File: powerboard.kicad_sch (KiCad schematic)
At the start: 27 parts, among them J1 B03B, J2 EMER_SW, J3 EMER_SW, Q1 TJ60S04M3L, U1 PQQ10W-Q24-S5-S, U2 TLP222A

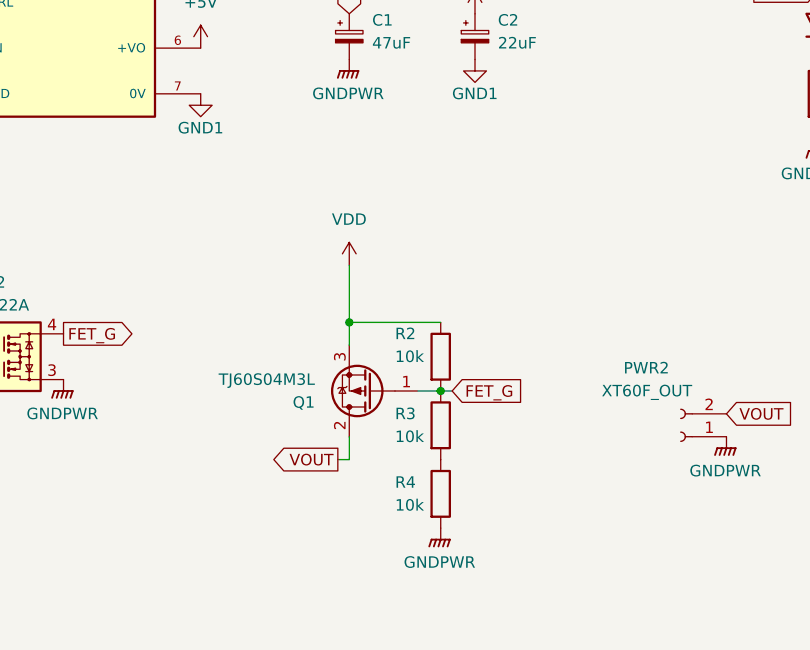
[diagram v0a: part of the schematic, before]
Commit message: ツェナーで定電圧チャレンジ
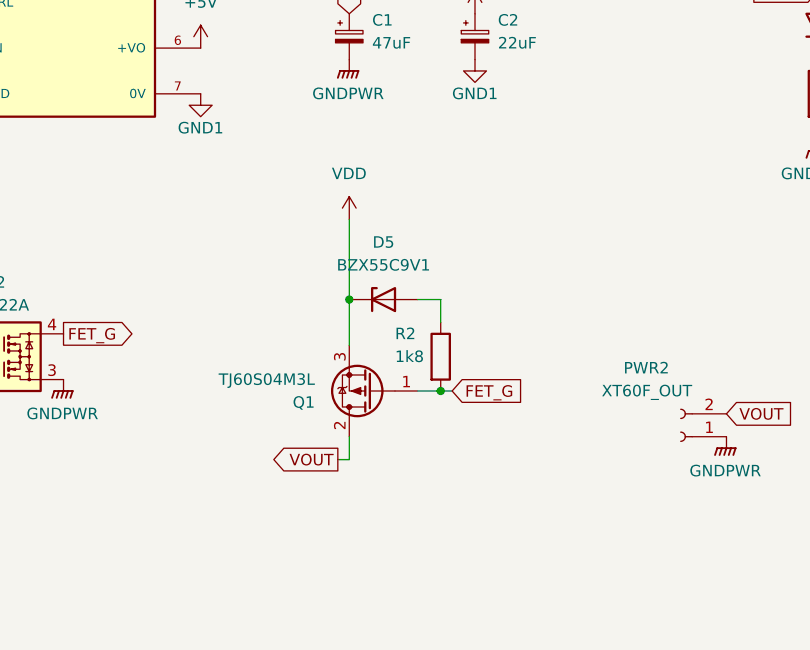
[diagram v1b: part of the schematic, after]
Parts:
- removed R3, R4: 10k, Resistor_THT:R_Axial_DIN0207_L6.3mm_D2.5mm_P7.62mm_Horizontal, symbol Device:R
- added D5: BZX55C9V1, Diode_THT:D_DO-35_SOD27_P10.16mm_Horizontal, symbol Diode:ZPDxx
- R2: value 10k -> 1k8
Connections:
- net VDD: now also D5.1 (K); no longer R2.1
- new net: D5.2 (A), R2.1
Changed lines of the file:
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@@
 	(paper "A4")
+	(junction
+		(at 144.78 66.04)
+		(diameter 0)
+		(color 0 0 0 0)
+	)
 	(junction
 		(at 154.94 76.2)
@@
 		(color 0 0 0 0)
 	)
-	(junction
-		(at 144.78 68.58)
-		(diameter 0)
-		(color 0 0 0 0)
-	)
 	(no_connect
 		(at 97.79 33.02)
@@
 	(wire
 		(pts
-			(xy 144.78 62.23) (xy 144.78 68.58)
+			(xy 144.78 57.15) (xy 144.78 66.04)
 		)
 		(stroke
@@
 	(wire
 		(pts
-			(xy 144.78 68.58) (xy 144.78 71.12)
+			(xy 55.88 41.91) (xy 39.37 41.91)
 		)
 		(stroke
@@
 	(wire
 		(pts
-			(xy 55.88 41.91) (xy 39.37 41.91)
+			(xy 67.31 69.85) (xy 80.01 69.85)
 		)
 		(stroke
@@
 	(wire
 		(pts
-			(xy 67.31 69.85) (xy 80.01 69.85)
+			(xy 82.55 69.85) (xy 86.36 69.85)
 		)
 		(stroke
@@
 	(wire
 		(pts
-			(xy 82.55 69.85) (xy 86.36 69.85)
+			(xy 96.52 38.1) (xy 97.79 38.1)
 		)
 		(stroke
@@
 	(wire
 		(pts
-			(xy 96.52 38.1) (xy 97.79 38.1)
+			(xy 97.79 74.93) (xy 97.79 77.47)
 		)
 		(stroke
@@
 	(wire
 		(pts
-			(xy 97.79 74.93) (xy 97.79 77.47)
+			(xy 60.96 39.37) (xy 59.69 39.37)
 		)
 		(stroke
@@
 	(wire
 		(pts
-			(xy 60.96 39.37) (xy 59.69 39.37)
+			(xy 25.4 71.12) (xy 33.02 71.12)
 		)
 		(stroke
@@
 	(wire
 		(pts
-			(xy 25.4 71.12) (xy 33.02 71.12)
+			(xy 55.88 41.91) (xy 55.88 43.18)
 		)
 		(stroke
@@
 	(wire
 		(pts
-			(xy 55.88 41.91) (xy 55.88 43.18)
+			(xy 144.78 83.82) (xy 144.78 81.28)
 		)
 		(stroke
@@
 	(wire
 		(pts
-			(xy 144.78 83.82) (xy 144.78 81.28)
+			(xy 156.21 76.2) (xy 154.94 76.2)
 		)
 		(stroke
@@
 	(wire
 		(pts
-			(xy 156.21 76.2) (xy 154.94 76.2)
+			(xy 96.52 44.45) (xy 96.52 43.18)
 		)
 		(stroke
@@
 	(wire
 		(pts
-			(xy 96.52 44.45) (xy 96.52 43.18)
+			(xy 152.4 66.04) (xy 154.94 66.04)
 		)
 		(stroke
@@
 	(wire
 		(pts
-			(xy 144.78 68.58) (xy 154.94 68.58)
+			(xy 144.78 66.04) (xy 144.78 71.12)
 		)
 		(stroke
@@
 		)
 	)
+	(wire
+		(pts
+			(xy 154.94 66.04) (xy 154.94 68.58)
+		)
+		(stroke
+			(width 0)
+			(type default)
+		)
+	)
 	(global_label "sig"
 		(shape input)
@@
 	)
 	(symbol
-		(lib_id "power:GNDPWR")
-		(at 154.94 91.44 0)
-		(unit 1)
-		(exclude_from_sim no)
-		(in_bom yes)
-		(on_board yes)
-		(dnp no)
-		(fields_autoplaced yes)
-		(property "Reference" "#PWR012"
-			(at 154.94 96.52 0)
-			(effects
-				(font
-					(size 1.27 1.27)
-				)
-				(hide yes)
-			)
-		)
-		(property "Value" "GNDPWR"
-			(at 154.813 95.25 0)
-			(effects
-				(font
-					(size 1.27 1.27)
-				)
-			)
-		)
-		(property "Footprint" ""
-			(at 154.94 92.71 0)
-			(effects
-				(font
-					(size 1.27 1.27)
-				)
-				(hide yes)
-			)
-		)
-		(property "Datasheet" ""
-			(at 154.94 92.71 0)
-			(effects
-				(font
-					(size 1.27 1.27)
-				)
-				(hide yes)
-			)
-		)
-		(property "Description" "Power symbol creates a global label with name \"GNDPWR\" , global ground"
-			(at 154.94 91.44 0)
-			(effects
-				(font
-					(size 1.27 1.27)
-				)
-				(hide yes)
-			)
-		)
-		(pin "1"
-		)
-		(instances
-			(project "powerboard"
-				(path "/f61afb78-be8f-4a5f-ad16-61c0881e4198"
-					(reference "#PWR012")
-					(unit 1)
-				)
-			)
-		)
-	)
-	(symbol
 		(lib_id "Connector:Conn_01x02_Socket")
 		(at 181.61 81.28 180)
@@
 	(symbol
 		(lib_id "power:VDD")
-		(at 144.78 62.23 0)
+		(at 144.78 57.15 0)
 		(unit 1)
 		(exclude_from_sim no)
@@
 		(fields_autoplaced yes)
 		(property "Reference" "#PWR011"
-			(at 144.78 66.04 0)
+			(at 144.78 60.96 0)
 			(effects
 				(font
@@
 		)
 		(property "Value" "VDD"
+			(at 144.78 52.07 0)
+			(effects
+				(font
+					(size 1.27 1.27)
+				)
+			)
+		)
+		(property "Footprint" ""
 			(at 144.78 57.15 0)
 			(effects
@@
 					(size 1.27 1.27)
 				)
-			)
-		)
-		(property "Footprint" ""
-			(at 144.78 62.23 0)
-			(effects
-				(font
-					(size 1.27 1.27)
-				)
 				(hide yes)
 			)
 		)
 		(property "Datasheet" ""
-			(at 144.78 62.23 0)
+			(at 144.78 57.15 0)
 			(effects
 				(font
@@
 		)
 		(property "Description" "Power symbol creates a global label with name \"VDD\""
-			(at 144.78 62.23 0)
+			(at 144.78 57.15 0)
 			(effects
 				(font
@@
 	)
 	(symbol
-		(lib_id "Device:R")
-		(at 154.94 87.63 0)
-		(unit 1)
-		(exclude_from_sim no)
-		(in_bom yes)
-		(on_board yes)
-		(dnp no)
-		(property "Reference" "R4"
-			(at 149.86 86.36 0)
-			(effects
-				(font
-					(size 1.27 1.27)
-				)
-				(justify left)
-			)
-		)
-		(property "Value" "10k"
-			(at 149.86 88.9 0)
-			(effects
-				(font
-					(size 1.27 1.27)
-				)
-				(justify left)
-			)
-		)
-		(property "Footprint" "Resistor_THT:R_Axial_DIN0207_L6.3mm_D2.5mm_P7.62mm_Horizontal"
-			(at 153.162 87.63 90)
-			(effects
-				(font
-					(size 1.27 1.27)
-				)
-				(hide yes)
-			)
-		)
-		(property "Datasheet" "~"
-			(at 154.94 87.63 0)
-			(effects
-				(font
-					(size 1.27 1.27)
-				)
-				(hide yes)
-			)
-		)
-		(property "Description" "Resistor"
-			(at 154.94 87.63 0)
-			(effects
-				(font
-					(size 1.27 1.27)
-				)
-				(hide yes)
-			)
-		)
-		(pin "1"
-		)
-		(pin "2"
-		)
-		(instances
-			(project "powerboard"
-				(path "/f61afb78-be8f-4a5f-ad16-61c0881e4198"
-					(reference "R4")
-					(unit 1)
-				)
-			)
-		)
-	)
-	(symbol
 		(lib_id "power:GNDPWR")
 		(at 96.52 44.45 0)
@@
 	)
 	(symbol
-		(lib_id "Device:R")
-		(at 154.94 80.01 0)
-		(unit 1)
-		(exclude_from_sim no)
-		(in_bom yes)
-		(on_board yes)
-		(dnp no)
-		(property "Reference" "R3"
-			(at 149.86 78.74 0)
-			(effects
-				(font
-					(size 1.27 1.27)
-				)
-				(justify left)
-			)
-		)
-		(property "Value" "10k"
-			(at 149.86 81.28 0)
-			(effects
-				(font
-					(size 1.27 1.27)
-				)
-				(justify left)
-			)
-		)
-		(property "Footprint" "Resistor_THT:R_Axial_DIN0207_L6.3mm_D2.5mm_P7.62mm_Horizontal"
-			(at 153.162 80.01 90)
-			(effects
-				(font
-					(size 1.27 1.27)
-				)
-				(hide yes)
-			)
-		)
-		(property "Datasheet" "~"
-			(at 154.94 80.01 0)
-			(effects
-				(font
-					(size 1.27 1.27)
-				)
-				(hide yes)
-			)
-		)
-		(property "Description" "Resistor"
-			(at 154.94 80.01 0)
-			(effects
-				(font
-					(size 1.27 1.27)
-				)
-				(hide yes)
-			)
-		)
-		(pin "1"
-		)
-		(pin "2"
-		)
-		(instances
-			(project "powerboard"
-				(path "/f61afb78-be8f-4a5f-ad16-61c0881e4198"
-					(reference "R3")
-					(unit 1)
-				)
-			)
-		)
-	)
-	(symbol
 		(lib_id "power:PWR_FLAG")
 		(at 252.73 67.31 180)
@@
 	)
 	(symbol
+		(lib_id "Diode:ZPDxx")
+		(at 148.59 66.04 0)
+		(unit 1)
+		(exclude_from_sim no)
+		(in_bom yes)
+		(on_board yes)
+		(dnp no)
+		(fields_autoplaced yes)
+		(property "Reference" "D5"
+			(at 148.59 59.69 0)
+			(effects
+				(font
+					(size 1.27 1.27)
+				)
+			)
+		)
+		(property "Value" "BZX55C9V1"
+			(at 148.59 62.23 0)
+			(effects
+				(font
+					(size 1.27 1.27)
+				)
+			)
+		)
+		(property "Footprint" "Diode_THT:D_DO-35_SOD27_P10.16mm_Horizontal"
+			(at 148.59 70.485 0)
+			(effects
+				(font
+					(size 1.27 1.27)
+				)
+				(hide yes)
+			)
+		)
+		(property "Datasheet" "http://diotec.com/tl_files/diotec/files/pdf/datasheets/zpd1"
+			(at 148.59 66.04 0)
+			(effects
+				(font
+					(size 1.27 1.27)
+				)
+				(hide yes)
+			)
+		)
+		(property "Description" "500mW Zener Diode, DO-35"
+			(at 148.59 66.04 0)
+			(effects
+				(font
+					(size 1.27 1.27)
+				)
+				(hide yes)
+			)
+		)
+		(pin "2"
+		)
+		(pin "1"
+		)
+		(instances
+			(project ""
+				(path "/f61afb78-be8f-4a5f-ad16-61c0881e4198"
+					(reference "D5")
+					(unit 1)
+				)
+			)
+		)
+	)
+	(symbol
 		(lib_id "Device:R")
 		(at 154.94 72.39 0)
@@
 			)
 		)
-		(property "Value" "10k"
+		(property "Value" "1k8"
 			(at 149.86 72.39 0)
 			(effects
